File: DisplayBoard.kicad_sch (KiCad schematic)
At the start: 0 parts

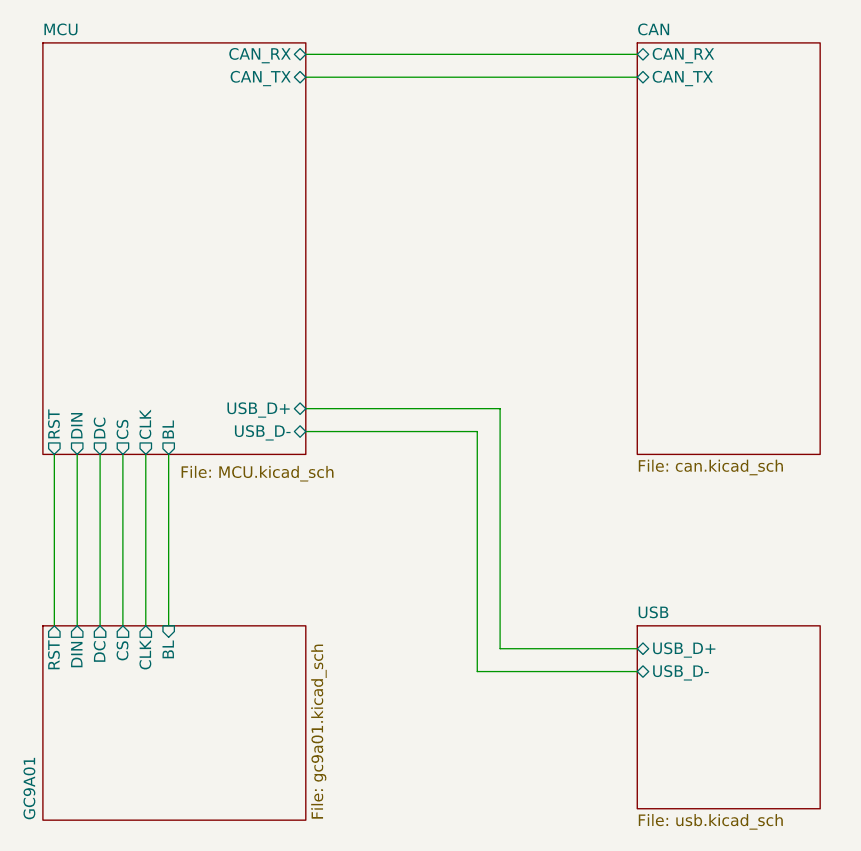
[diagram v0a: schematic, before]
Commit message: Finished v1.1
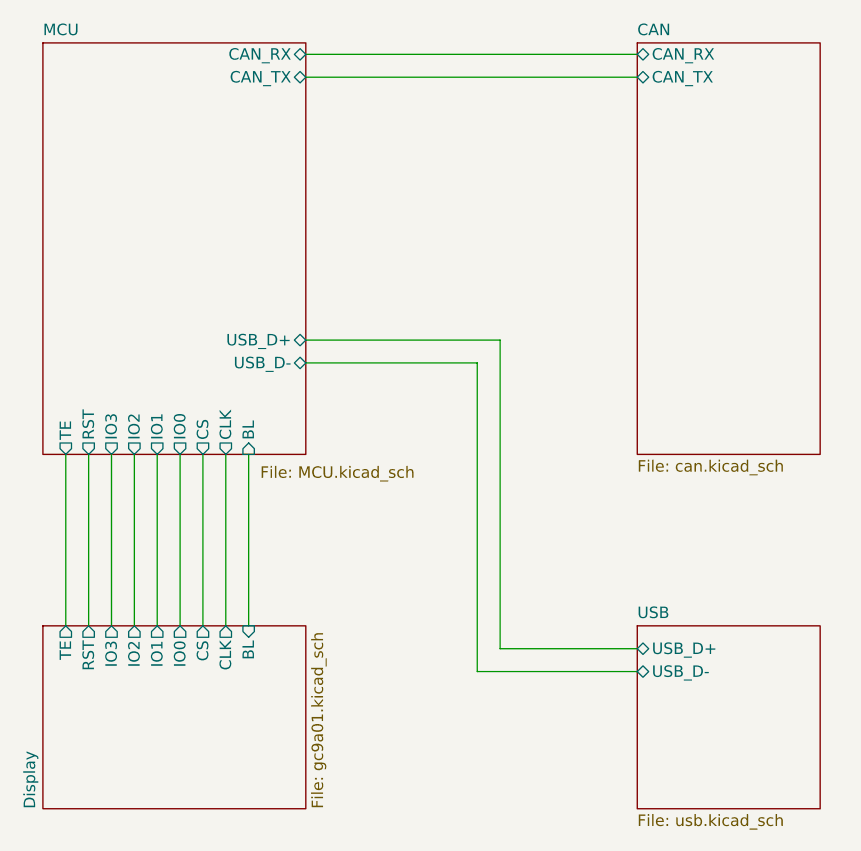
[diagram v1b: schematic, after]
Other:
- sheet GC9A01 renamed Display
- sheet Display ports: added IO0, IO1, IO2, IO3, TE; removed DC, DIN
- sheet MCU ports: added IO0, IO1, IO2, IO3, TE; removed DC, DIN
